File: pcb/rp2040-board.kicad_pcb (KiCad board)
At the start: 4 copper layers, 150 x 71 mm, 52 parts, among them J1 DMX, J1 RS485, J2 GPIO, J3 ELRS, J4 OLED, J5 SWD, J6 USB_C_Receptacle_USB2.0_16P, SW1 USB Boot, SW2 RotaryEncoder_Switch, SW3 Reset, U1 W25Q128JVS, U2 SP485EEN-L/TR, U3 RP2040, U4 AMS1117-3.3, Y1 12MHz

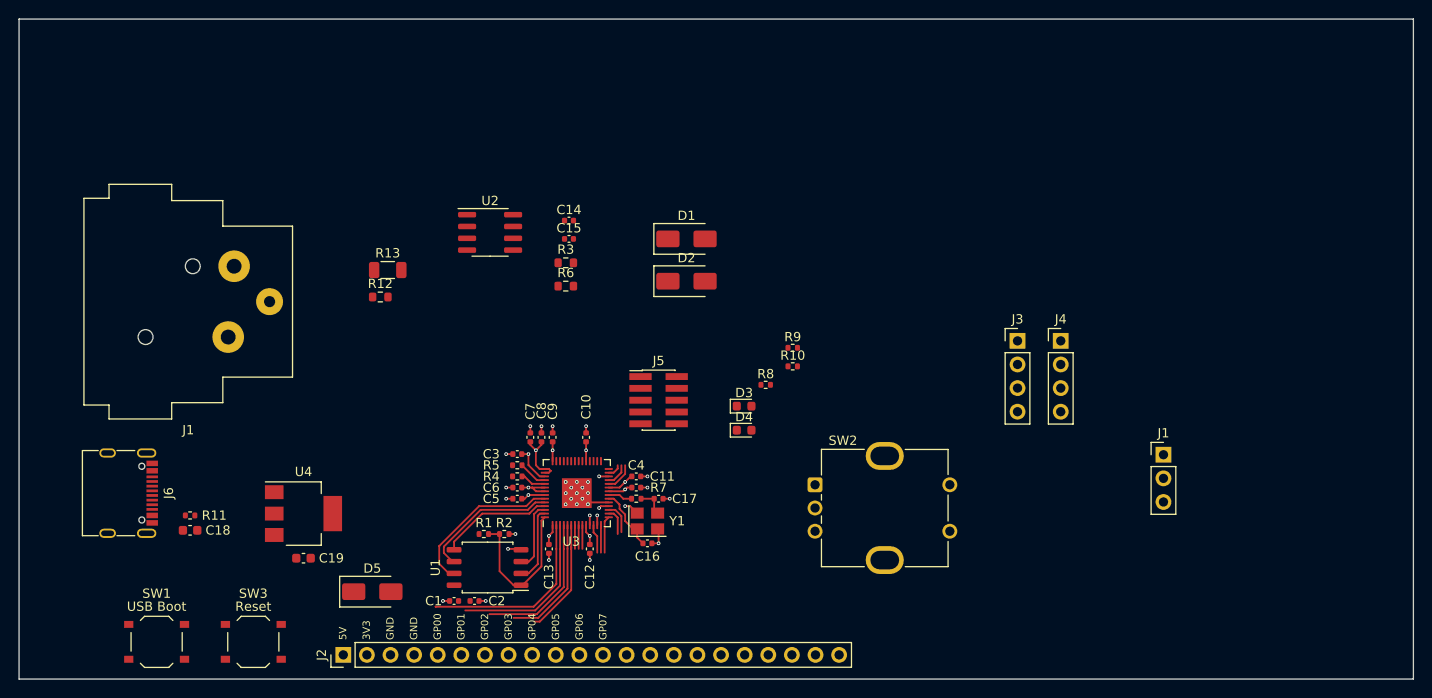
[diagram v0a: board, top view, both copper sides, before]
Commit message: board wip
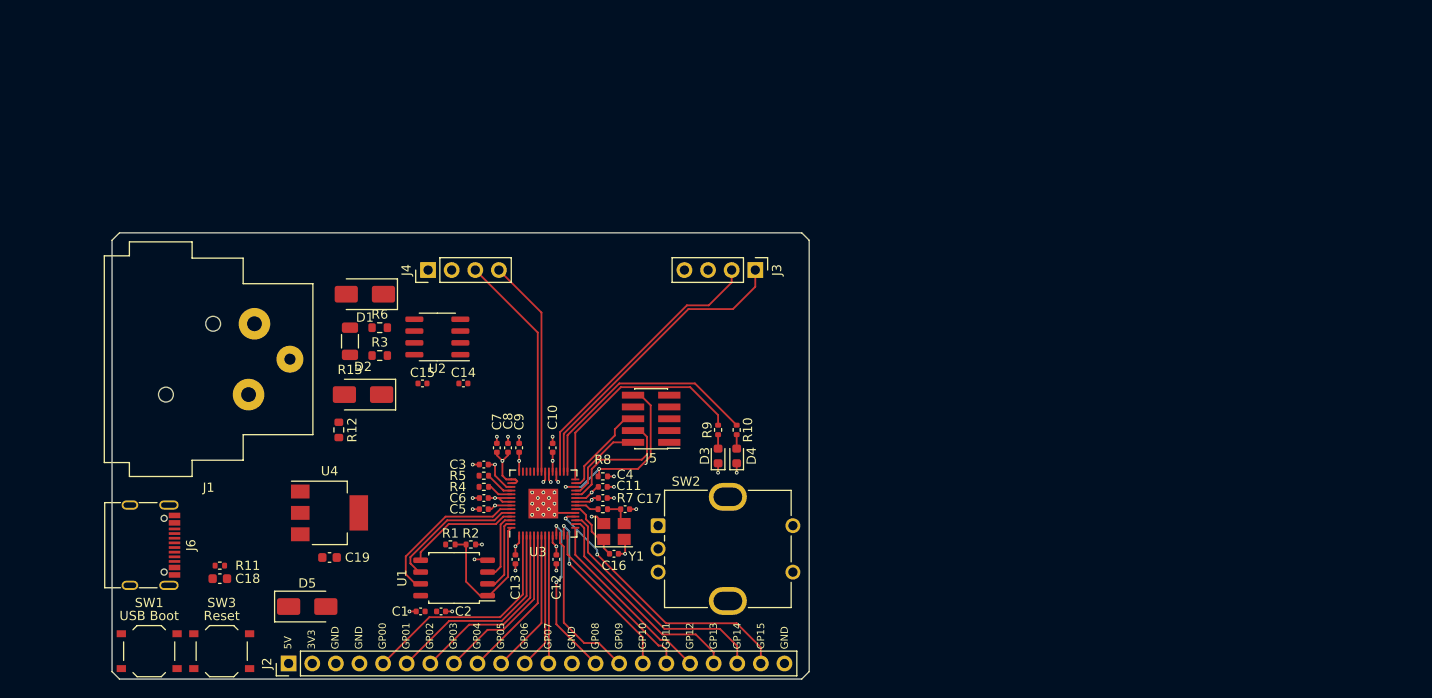
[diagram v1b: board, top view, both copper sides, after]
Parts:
- removed the J1 at (213.1, 95.9)
- moved J4 68.5 mm to (134.0, 76.0), turned to 90 degrees
- moved D2 36.9 mm to (127.0, 89.4), turned to 180 degrees
- moved D1 35.1 mm to (127.2, 78.6), turned to 180 degrees
- moved J3 29.2 mm to (169.2, 76.0), turned to -90 degrees
- moved R3 22.4 mm to (128.8, 85.2)
- moved C15 22.1 mm to (133.4, 88.2)
- moved C14 20.9 mm to (137.8, 88.2)
- moved R6 20.5 mm to (128.8, 82.2)
- moved R8 20.1 mm to (152.8, 98.2)
- moved SW2 17.4 mm to (158.8, 103.5)
- moved R12 15.0 mm to (124.4, 93.2), turned to -90 degrees
- moved U2 12.6 mm to (135.0, 83.2), turned to 180 degrees
- moved R9 11.9 mm to (165.2, 93.2), turned to 90 degrees
- moved R10 9.12 mm to (167.2, 93.2), turned to 90 degrees
- moved R13 8.67 mm to (125.6, 83.7), turned to 90 degrees
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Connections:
- U3 pad 28: OLED_SCK -> LED_D1
- U3 pad 29: OLED_SDA -> LED_D2
- U3 pad 36: LED_D2 -> OLED_SDA
- U3 pad 37: LED_D1 -> OLED_SCK
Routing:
- net ELRS_TX: track 0.00 -> 33.0 mm
- net ELRS_RX: track 0.00 -> 30.7 mm
- net GPIO15: track 1.12 -> 29.9 mm, vias 1 -> 2
- net LED_D2: track 0.00 -> 26.3 mm
- net LED_D1: track 0.00 -> 24.7 mm
- net OLED_SCK: track 0.00 -> 24.5 mm
- net OLED_SDA: track 0.00 -> 23.6 mm
- net GPIO14: track 3.37 -> 26.5 mm
- net GPIO13: track 2.91 -> 23.6 mm
- net RUN: track 1.04 -> 21.1 mm, vias 1 -> 2
- net GPIO10: track 1.04 -> 19.4 mm, vias 1 -> 2
- net GPIO08: track 1.04 -> 18.0 mm, vias 1 -> 2
- net GPIO12: track 3.98 -> 20.1 mm
- net GPIO11: track 2.96 -> 18.4 mm
- net GPIO09: track 3.13 -> 17.3 mm
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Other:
- board size 150 x 71 mm -> 75 x 48 mm
- board text added: "5V 3V3 GND GND GP00 GP01 GP02 GP03 GP04 GP05 GP06 GP07 GND GP08 GP09 GP10 GP11 GP12 GP13 GP14 GP15 GND"
- board text removed: "5V 3V3 GND GND GP00 GP01 GP02 GP03 GP04 GP05 GP06 GP07"
